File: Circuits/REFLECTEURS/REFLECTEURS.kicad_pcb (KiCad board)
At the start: 2 copper layers, 24 parts, among them P1 HE10-10, U1 3mm_hole, U2 3mm_hole

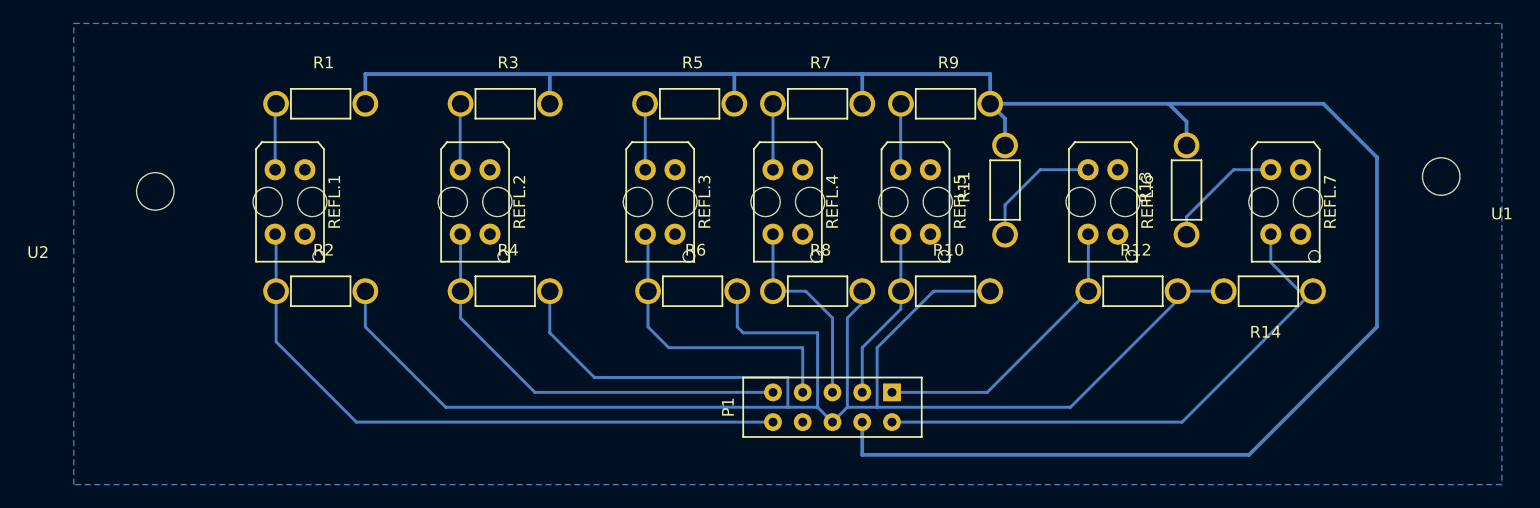
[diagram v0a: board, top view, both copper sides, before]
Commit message: Ameliorations cartes + rapport
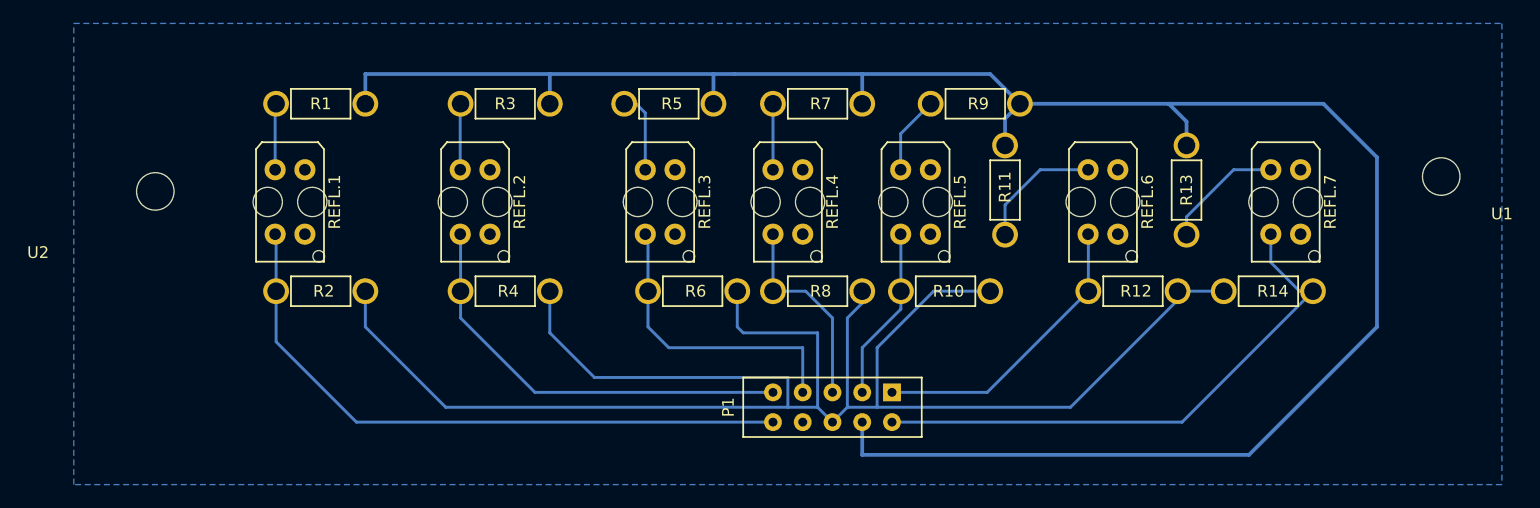
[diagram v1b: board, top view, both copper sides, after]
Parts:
- moved R9 2.54 mm to (94.7, 32.5)
- moved R5 1.78 mm to (68.6, 32.5)
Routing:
- net +5V: track 175.0 -> 173.5 mm
- net Net-(R5-Pad1): track 5.64 -> 7.00 mm
- net Net-(R9-Pad1): track 5.64 -> 6.72 mm
